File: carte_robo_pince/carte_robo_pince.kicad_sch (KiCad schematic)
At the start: 17 parts, among them J1 Conn_01x18_Pin, J2 Conn_01x18_Pin, J3 Conn_01x03_Socket, J4 Conn_01x03_Socket, J5 Conn_01x03_Socket, J6 Conn_01x03_Socket, J7 Conn_01x03_Socket, SW1 SW_DIP_x01, U1 KA78M05_TO252

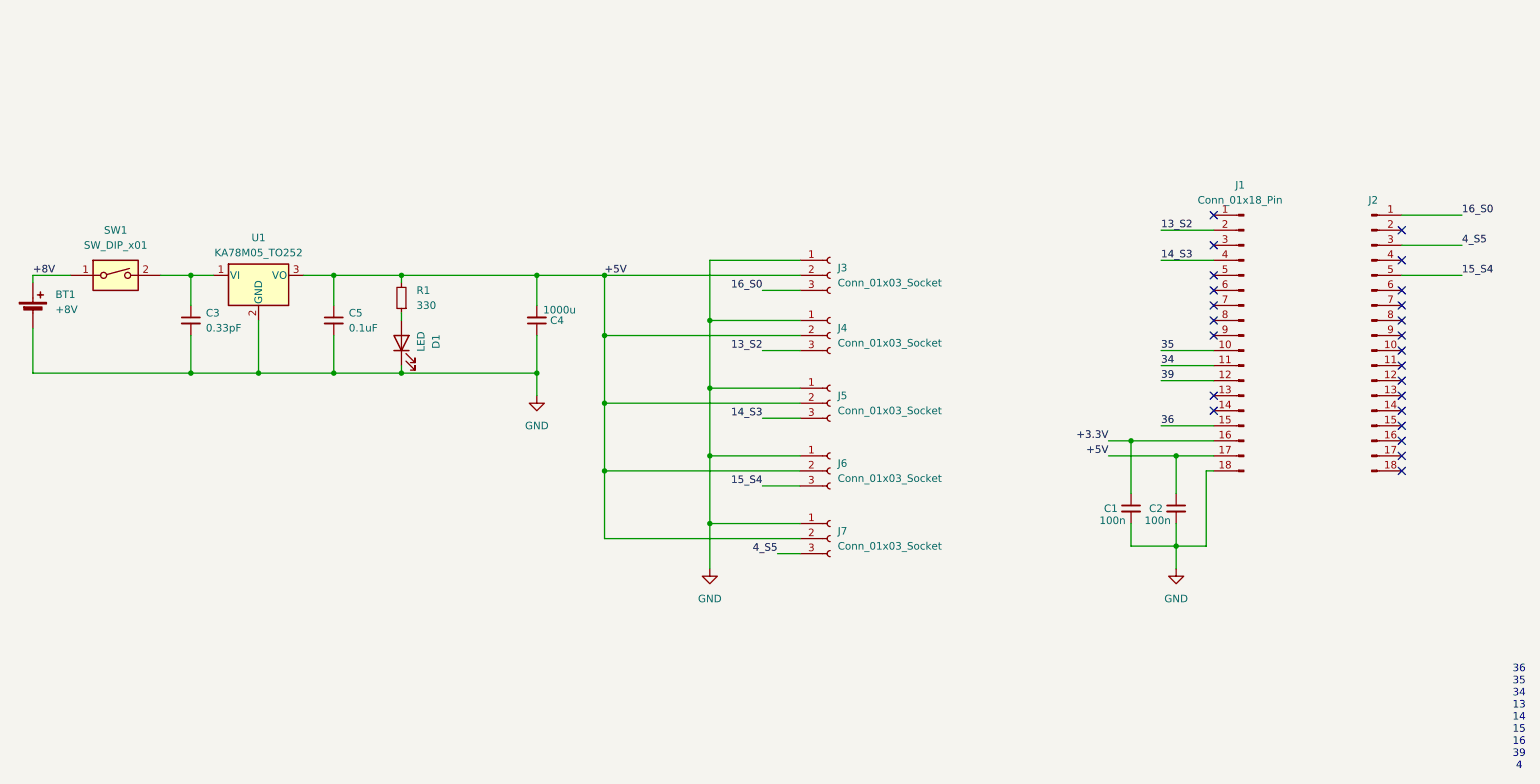
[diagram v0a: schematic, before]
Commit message: 01/04/25
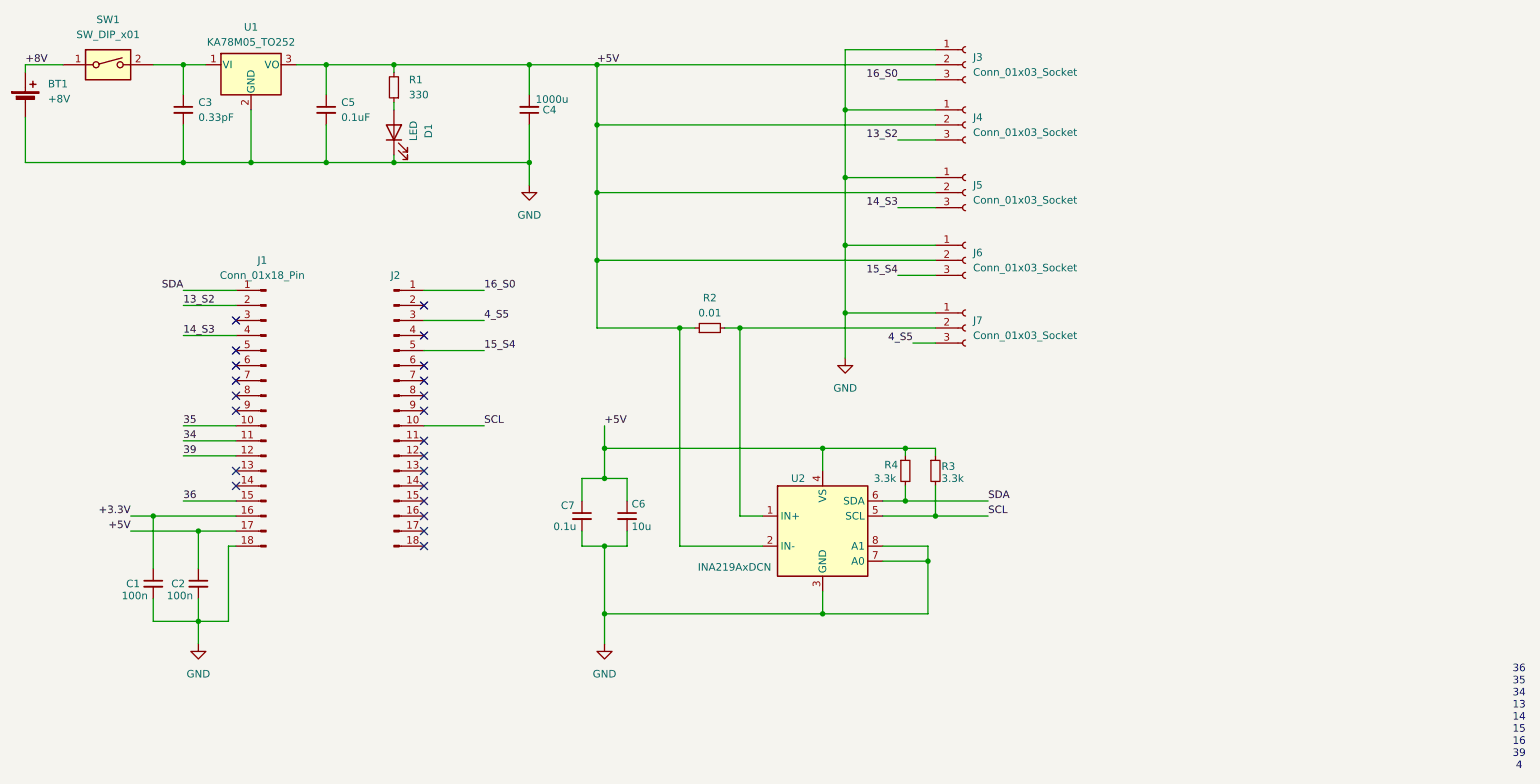
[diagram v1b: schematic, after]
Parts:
- added C6: 10u, Capacitor_THT:C_Disc_D3.0mm_W1.6mm_P2.50mm, symbol GW_Passives:C_Small
- added C7: 0.1u, Capacitor_THT:C_Disc_D3.0mm_W1.6mm_P2.50mm, symbol GW_Passives:C_Small
- added R2: 0.01, GW_Passives:R_2512_6332Metric, symbol GW_Passives:R_Small
- added R3, R4: 3.3k, Resistor_THT:R_Axial_DIN0207_L6.3mm_D2.5mm_P10.16mm_Horizontal, symbol GW_Passives:R_Small
- added U2: INA219AxDCN, Package_TO_SOT_SMD:SOT-23-8, symbol Sensor_Energy:INA219AxDCN
- SW1: footprint (none) -> Button_Switch_THT:SW_slide-03_P5_THT
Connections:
- net +5V: now also C6.1, C7.1, R2.1, R3.1, R4.1, U2.2 (IN-), U2.4 (VS); no longer J7.2 (Pin_2)
- net GND: now also C6.2, C7.2, U2.3 (GND), U2.7 (A0), U2.8 (A1)
- net SCL: now reaches J2.10 (Pin_10)
- net SCL: now also R3.2, U2.5 (SCL)
- net SDA: now reaches J1.1 (Pin_1)
- net SDA: now also R4.2, U2.6 (SDA)
- new net: J7.2 (Pin_2), R2.2, U2.1 (IN+)
- no-connect marks 24 -> 22
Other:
- moved on the sheet: BT1, C1, C2, C3, C4, C5, D1, J1, J2, J3, J4, J5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
